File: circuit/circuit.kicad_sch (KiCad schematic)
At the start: 23 parts

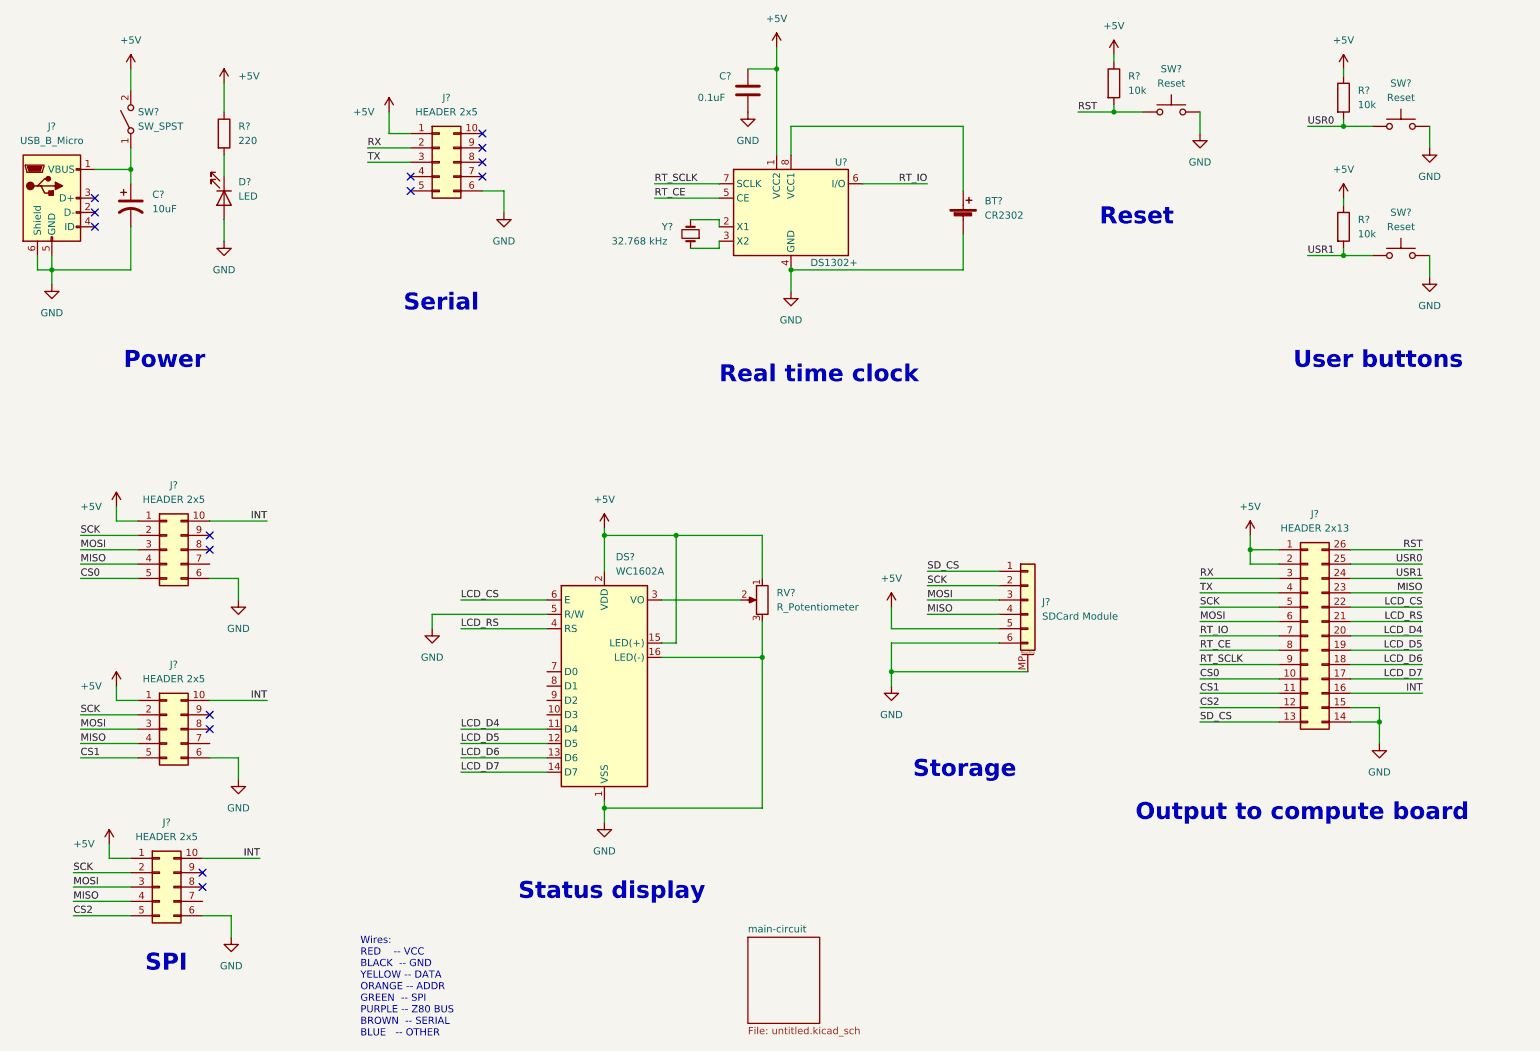
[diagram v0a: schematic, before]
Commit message: .
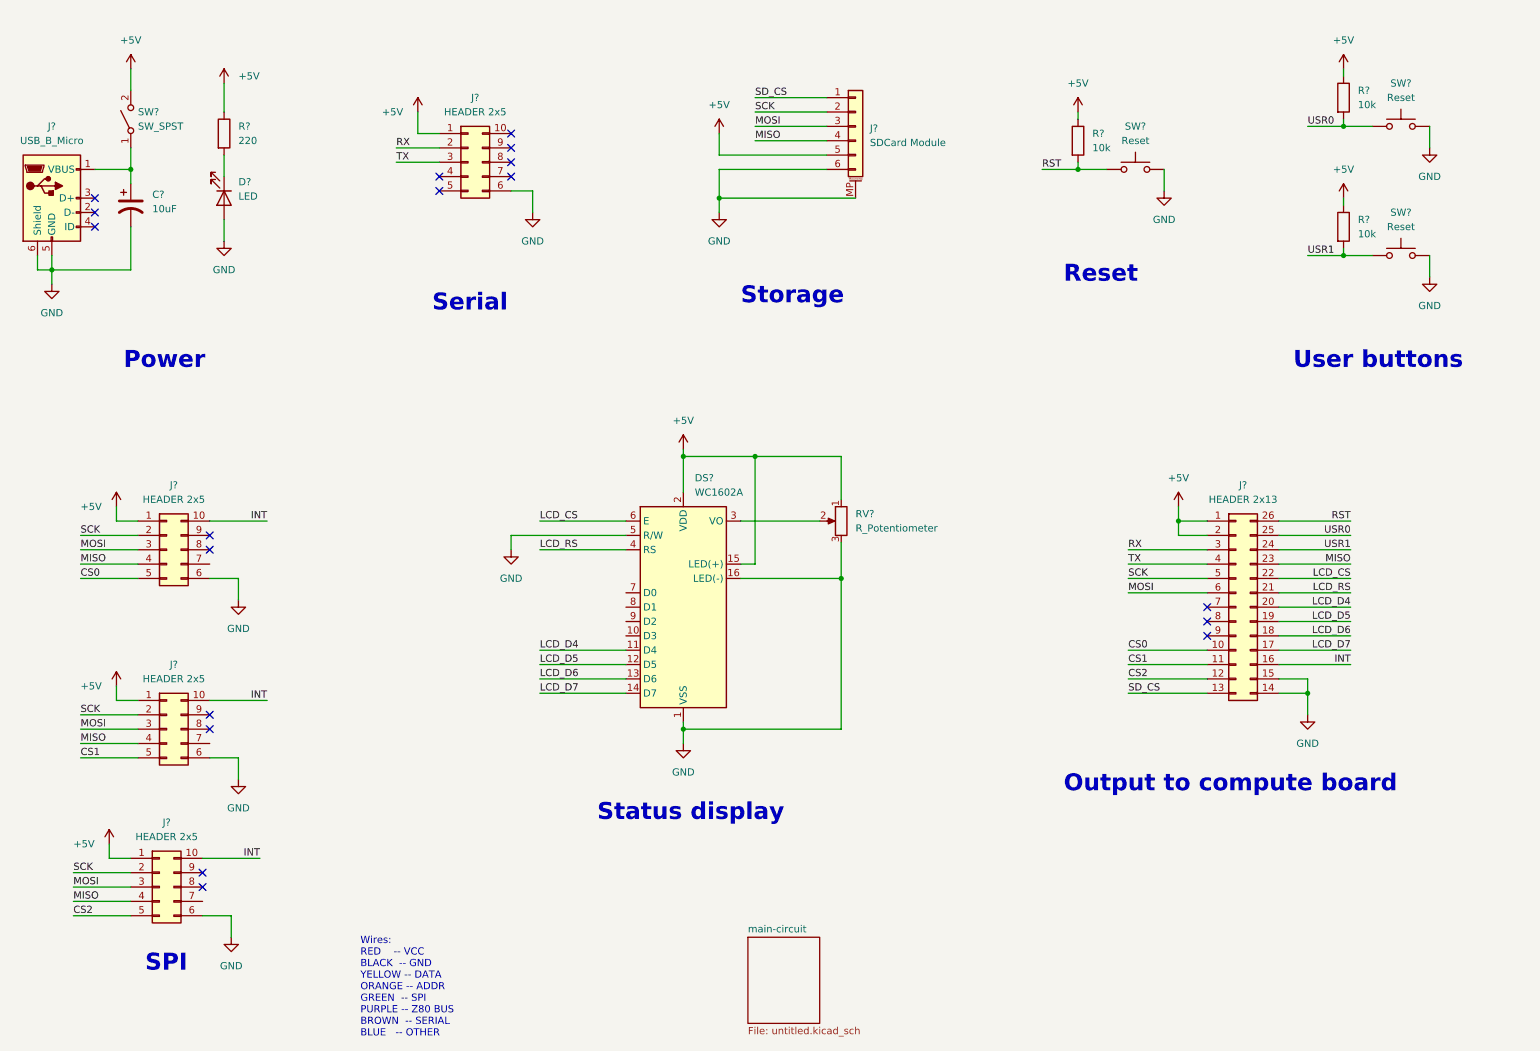
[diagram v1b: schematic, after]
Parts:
- removed BT?: CR2302, symbol Device:Battery_Cell
- removed C?: 0.1uF, symbol Device:C
- removed U?: DS1302+, Package_DIP:DIP-8_W7.62mm, symbol Timer_RTC:DS1302+
- removed Y?: 32.768 kHz, symbol Device:Crystal_Small
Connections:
- net RT_CE: no longer names the net of J?.8 (Pin_8)
- net RT_IO: no longer names the net of J?.7 (Pin_7)
- net RT_SCLK: no longer names the net of J?.9 (Pin_9)
- no-connect marks 15 -> 18
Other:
- note removed: "Real time clock"
- moved on the sheet: DS?, J?, R?, RV?, SW?

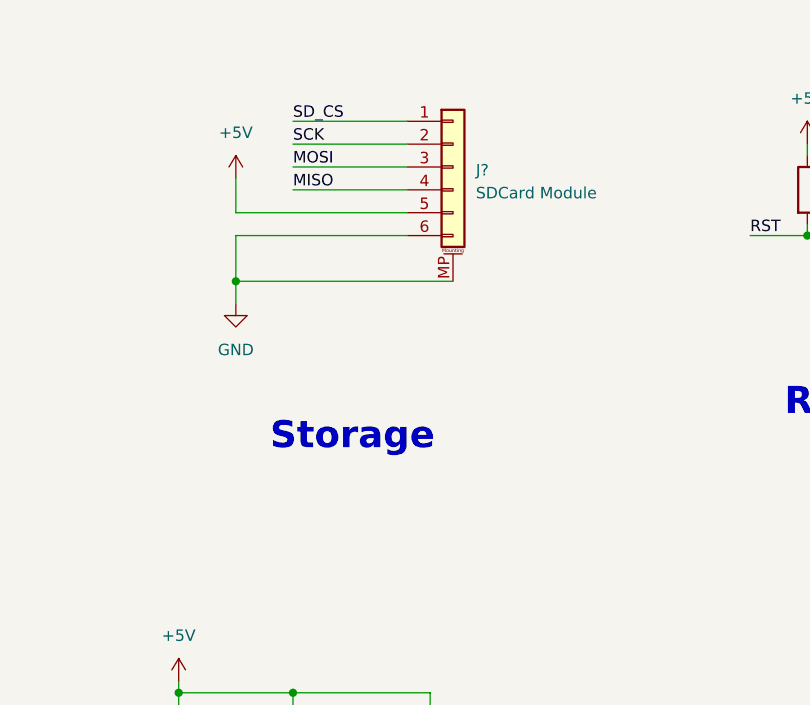
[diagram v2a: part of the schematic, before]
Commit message: .
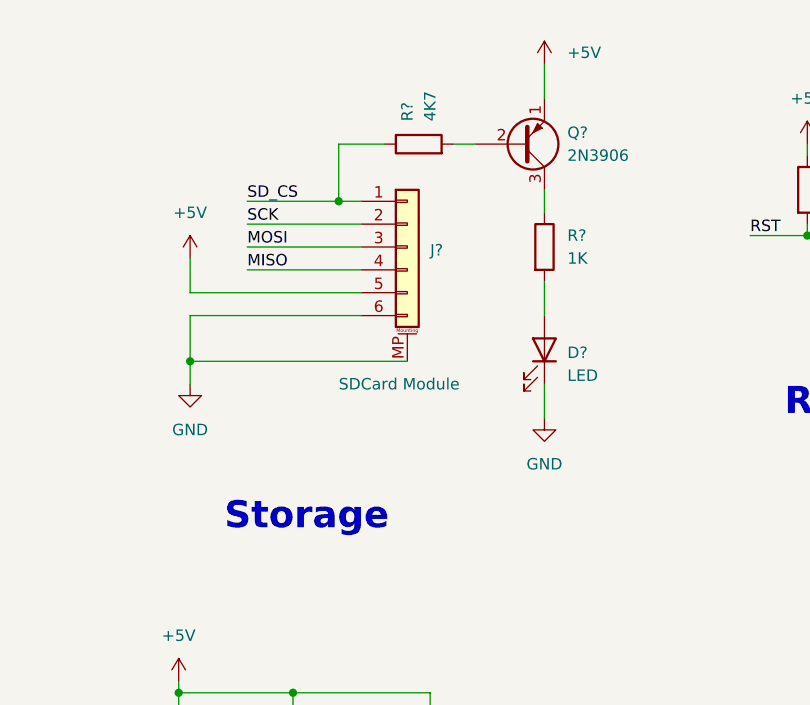
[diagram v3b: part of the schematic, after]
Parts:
- added D?: LED, symbol Device:LED
- added Q?: 2N3906, Package_TO_SOT_THT:TO-92_Inline, symbol Transistor_BJT:2N3906
- added R?: 1K, symbol Device:R
- added R?: 4K7, symbol Device:R
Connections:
- net +5V: now also Q?.1 (E)
- net GND: now also D?.1 (K)
- net SD_CS: now also R?.1
- new net: D?.2 (A), R?.2
- new net: Q?.3 (C), R?.1
- new net: Q?.2 (B), R?.2
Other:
- moved on the sheet: J?
